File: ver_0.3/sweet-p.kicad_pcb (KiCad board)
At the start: 2 copper layers, 84.3 x 76.2 mm, 50 parts, among them J1 Screw_Terminal_01x02, J2 Conn_01x11_Female, J3 Screw_Terminal_01x03, J4 Conn_01x08_Female, J5 Conn_01x06_Female, J6 Screw_Terminal_01x04, J7 Micro_SD_Card, U1 adafruit_tpl511x, U2 MCP1700-3302E_TO, U3 adafruit_ads1115, U4 ssd1306, U5 RFM95W-868S2, U6 Adafruit-Mini-GPS, U7 ds3231

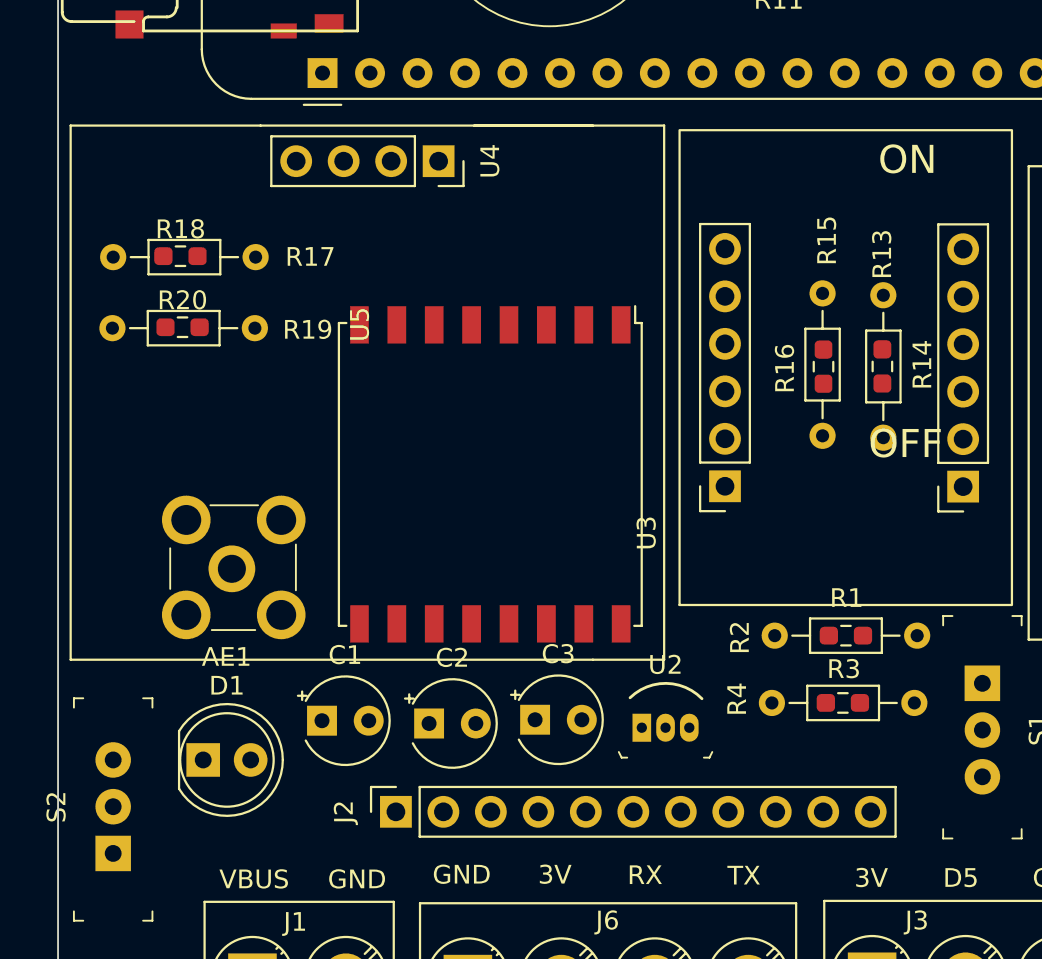
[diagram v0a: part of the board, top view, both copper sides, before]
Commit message: fixed breakout
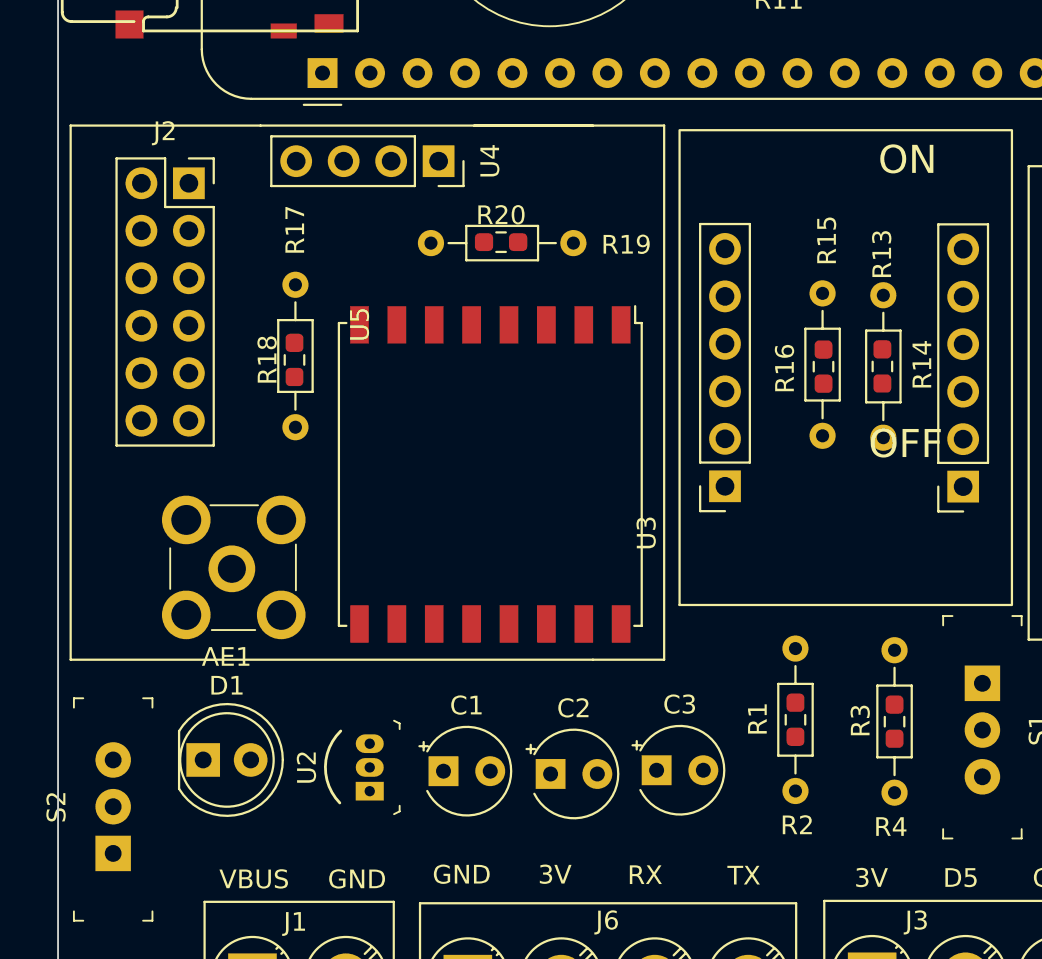
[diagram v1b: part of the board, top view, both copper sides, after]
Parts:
- J2: value Conn_01x11_Female -> Conn_01x12_Female; footprint Connector_PinSocket_2.54mm:PinSocket_1x11_P2.54mm_Vertical -> Connector_PinSocket_2.54mm:PinSocket_2x06_P2.54mm_Vertical
- moved J2 35.4 mm to (-5.05, 28.0), turned to 0 degrees
- moved R19 17.6 mm to (7.90, 31.2)
- moved R20 17.6 mm to (11.7, 31.1)
- moved U2 14.9 mm to (4.62, 60.5), turned to 90 degrees
- moved R17 13.3 mm to (0.65, 41.0), turned to 90 degrees
- moved R18 8.25 mm to (0.60, 37.5), turned to 90 degrees
- moved R4 8.13 mm to (32.7, 60.6), turned to 90 degrees
- moved C2 7.04 mm to (14.3, 59.6)
- moved C1 7.04 mm to (8.57, 59.5)
- moved C3 7.04 mm to (20.0, 59.4)
- moved R2 6.55 mm to (27.4, 52.9), turned to -90 degrees
- moved R1 5.25 mm to (27.4, 56.7), turned to -90 degrees
- moved R3 2.94 mm to (32.7, 56.8), turned to -90 degrees
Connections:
- U6 pad 1: GND_1 -> GND
